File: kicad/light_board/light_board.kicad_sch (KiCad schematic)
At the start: 34 parts, among them J1 24V, J10 Screw_Terminal_01x02, J11 Screw_Terminal_01x02, J12 VAC, J13 NEUTRAL, J14 GND, J17 MCU_GND, J2 GND, J3 MCU_L1, J4 MCU_L2, J5 MCU_L3, J6 MCU_Bike, J7 MCU_5V, J8 Screw_Terminal_01x02, J9 Screw_Terminal_01x02, K1 1462041-7, Q1 FDD8453LZ, Q2 FDD8453LZ, Q4 FDD8453LZ, Q5 MOCD207M, Q6 MOCD207M

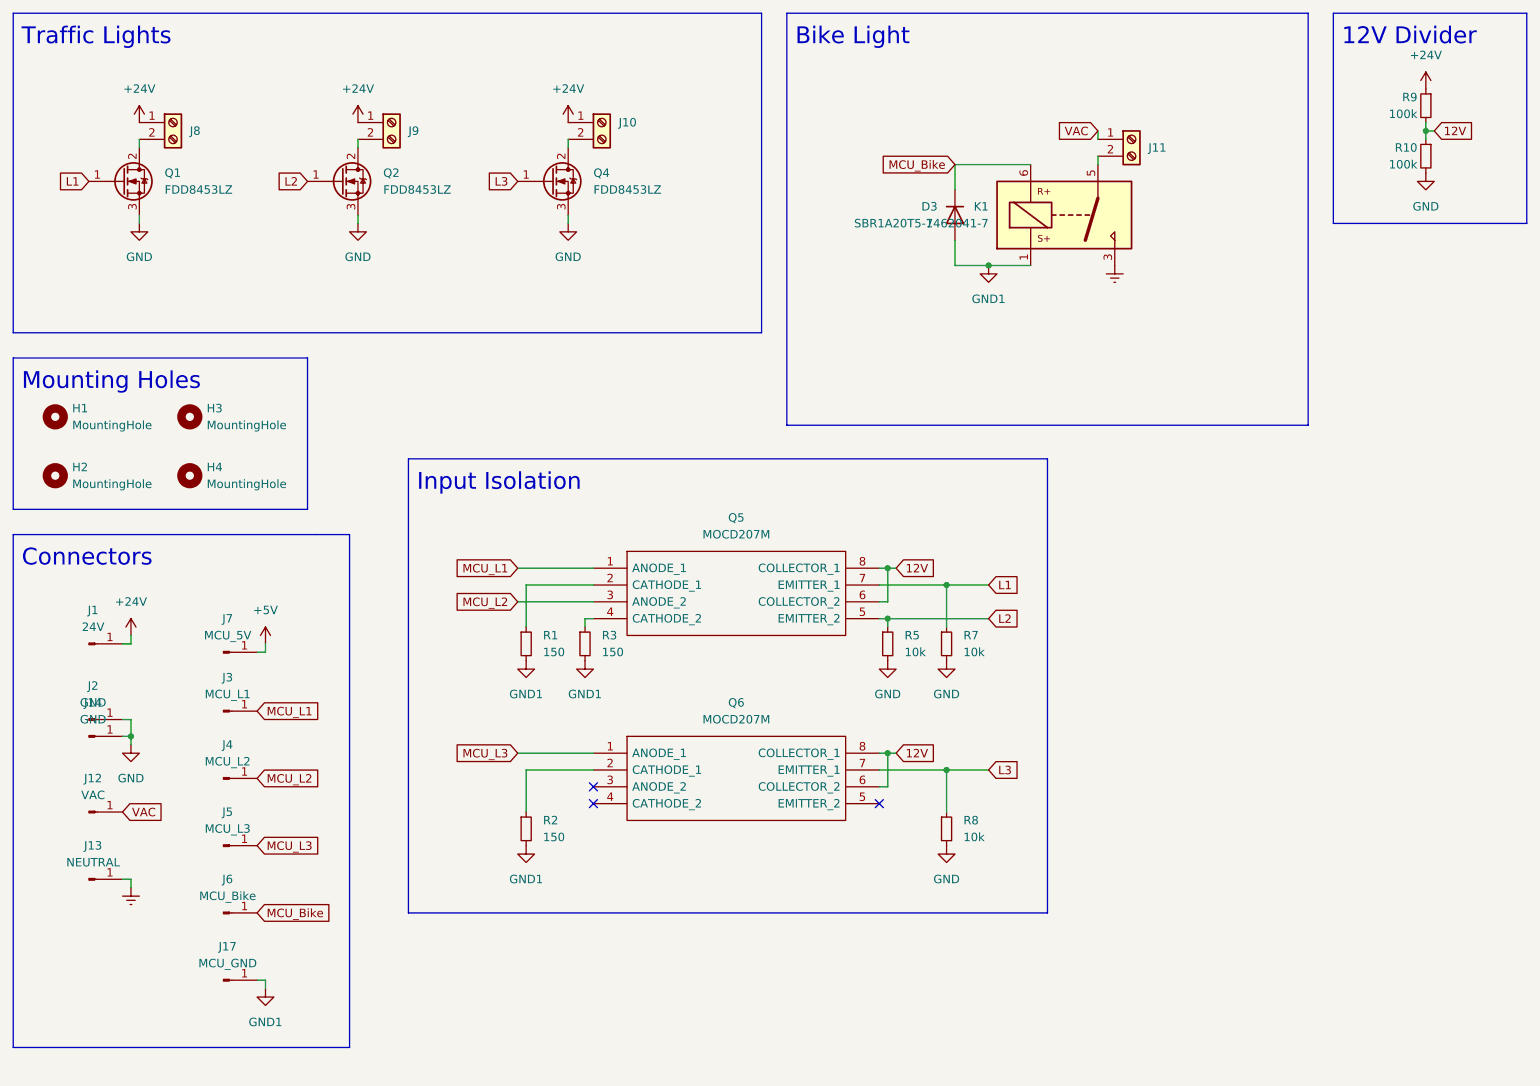
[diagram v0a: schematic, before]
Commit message: light board v2
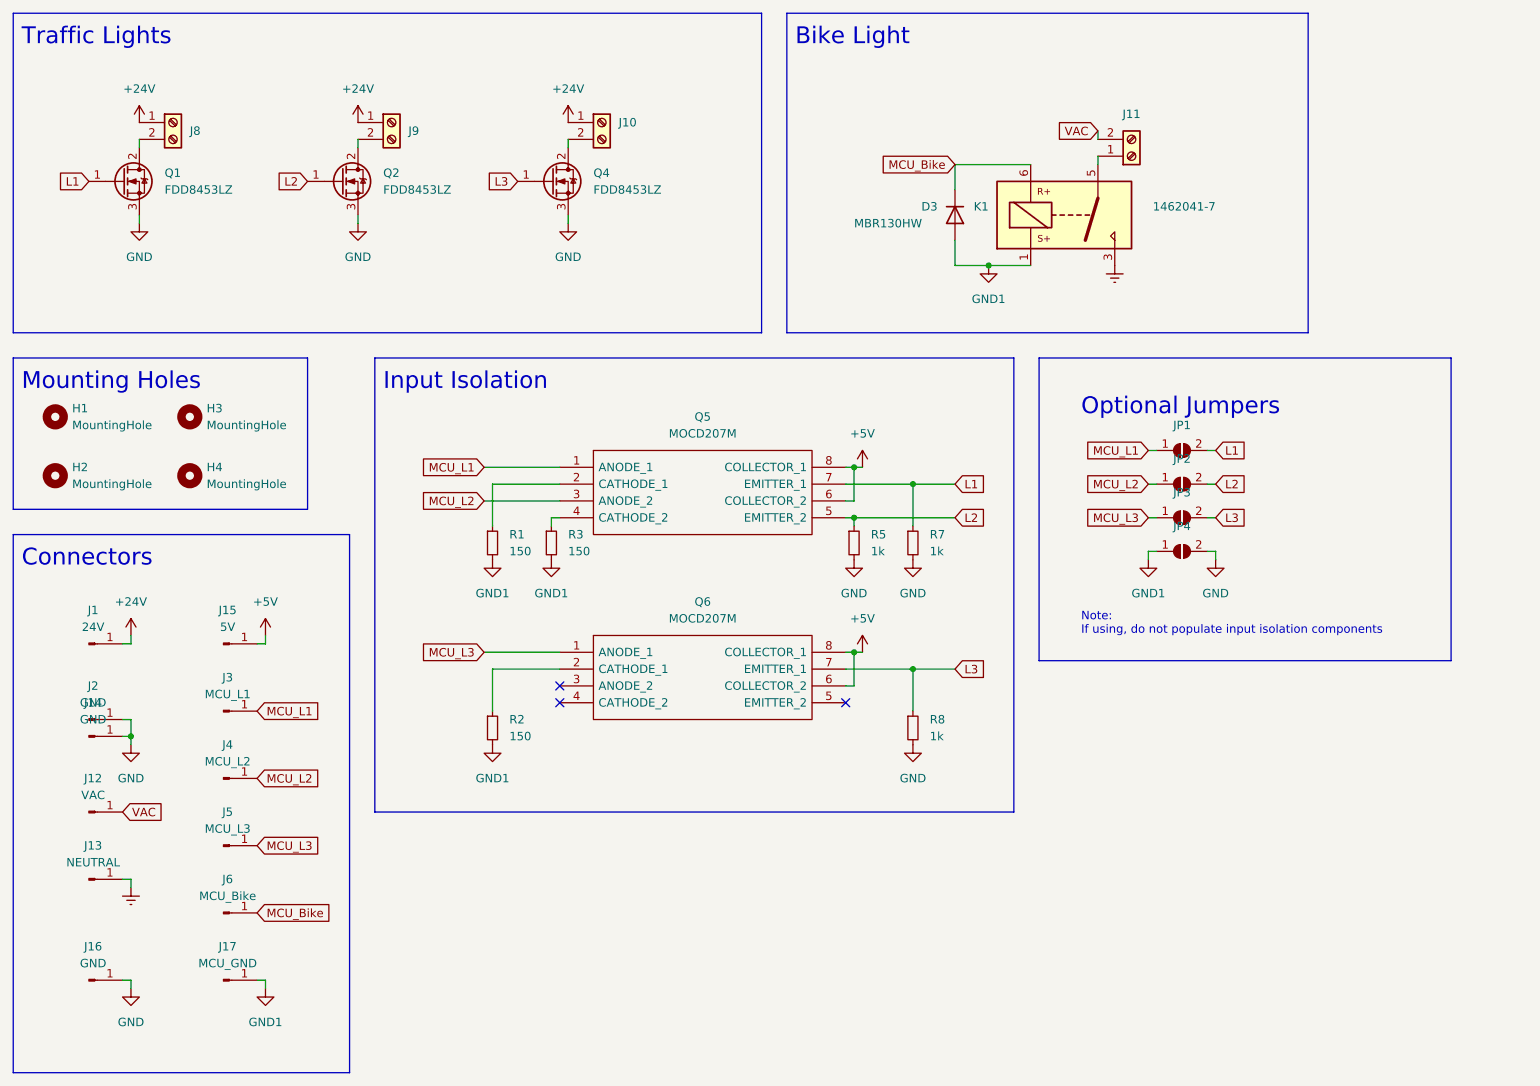
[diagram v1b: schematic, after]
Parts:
- removed J7: MCU_5V, Connector_PinHeader_2.54mm:PinHeader_1x01_P2.54mm_Vertical, symbol Connector:Conn_01x01_Male
- removed R10, R9: 100k, Resistor_SMD:R_1206_3216Metric, symbol Device:R_Small
- added J15: 5V, Connector_PinHeader_2.54mm:PinHeader_1x01_P2.54mm_Vertical, symbol Connector:Conn_01x01_Male
- added J16: GND, Connector_PinHeader_2.54mm:PinHeader_1x01_P2.54mm_Vertical, symbol Connector:Conn_01x01_Male
- added JP1, JP2, JP3, JP4: SolderJumper_2_Open, Jumper:SolderJumper-2_P1.3mm_Open_TrianglePad1.0x1.5mm, symbol Jumper:SolderJumper_2_Open
- D3: value SBR1A20T5-7 -> MBR130HW; footprint Diode_SMD:D_SOD-523 -> Diode_SMD:D_SOD-123
- R1, R2, R3: footprint Resistor_SMD:R_0805_2012Metric -> Resistor_SMD:R_0603_1608Metric
- R5, R7, R8: value 10k -> 1k; footprint Resistor_SMD:R_0805_2012Metric -> Resistor_SMD:R_0603_1608Metric
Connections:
- net 12V is gone; now on net +5V: Q5.6 (COLLECTOR_2), Q5.8 (COLLECTOR_1), Q6.6 (COLLECTOR_2), Q6.8 (COLLECTOR_1)
- net +5V: now also J15.1 (Pin_1)
- net GND: now also J16.1 (Pin_1), JP4.2 (B)
- net GND1: now also JP4.1 (A)
- net L1: now also JP1.2 (B)
- net L2: now also JP2.2 (B)
- net L3: now also JP3.2 (B)
- net MCU_L1: now also JP1.1 (A)
- net MCU_L2: now also JP2.1 (A)
- net MCU_L3: now also JP3.1 (A)
- net VAC: now also J11.2 (Pin_2); no longer J11.1 (Pin_1)
- net at K1.5: now also J11.1 (Pin_1); no longer J11.2 (Pin_2)
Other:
- note added: "Note: If using, do not populate input isolation components"
- note added: "Optional Jumpers"
- note removed: "12V Divider"
- moved on the sheet: Q5, Q6, R1, R2, R3, R5, R7, R8

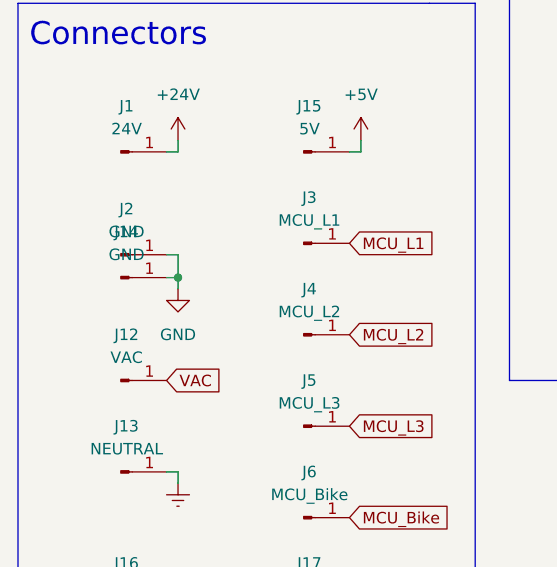
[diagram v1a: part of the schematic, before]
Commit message: update pcbs
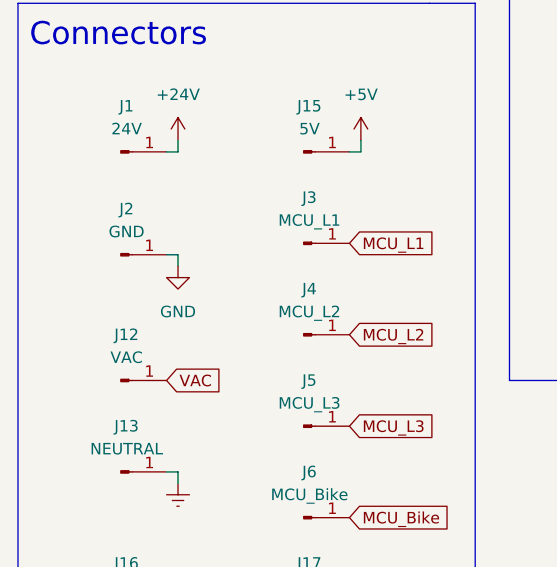
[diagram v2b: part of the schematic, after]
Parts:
- removed J14: GND, Connector_PinHeader_2.54mm:PinHeader_1x01_P2.54mm_Vertical, symbol Connector:Conn_01x01_Male
- J1, J12, J13, J2: footprint Connector_PinHeader_2.54mm:PinHeader_1x01_P2.54mm_Vertical -> _mylib:hole
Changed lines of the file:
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@@
   (junction (at 166.37 55.88) (diameter 0) (color 0 0 0 0)
-  )
-  (junction (at 36.83 127) (diameter 0) (color 0 0 0 0)
   )
   (junction (at 146.05 93.98) (diameter 0) (color 0 0 0 0)
@@
   (no_connect (at 144.78 121.92))
   (no_connect (at 101.6 119.38))
-  (wire (pts (xy 36.83 127) (xy 36.83 128.27))
-    (stroke (width 0) (type default) (color 0 0 0 0))
-  )
   (wire (pts (xy 146.05 86.36) (xy 144.78 86.36))
     (stroke (width 0) (type default) (color 0 0 0 0))
@@
     (stroke (width 0) (type default) (color 0 0 0 0))
   )
-  (wire (pts (xy 35.56 127) (xy 36.83 127))
-    (stroke (width 0) (type default) (color 0 0 0 0))
-  )
   (wire (pts (xy 146.05 93.98) (xy 146.05 95.25))
     (stroke (width 0) (type default) (color 0 0 0 0))
@@
     (stroke (width 0) (type default) (color 0 0 0 0))
   )
-  (wire (pts (xy 36.83 124.46) (xy 36.83 127))
+  (wire (pts (xy 36.83 124.46) (xy 36.83 125.73))
     (stroke (width 0) (type default) (color 0 0 0 0))
   )
@@
     (property "Reference" "J12" (id 0) (at 31.115 133.35 0))
     (property "Value" "VAC" (id 1) (at 31.115 135.89 0))
-    (property "Footprint" "Connector_PinHeader_2.54mm:PinHeader_1x01_P2.54mm_Vertical" (id 2) (at 30.48 138.43 0)
+    (property "Footprint" "_mylib:hole" (id 2) (at 30.48 138.43 0)
       (effects (font (size 1.27 1.27)) hide)
     )
@@
     (property "Reference" "J2" (id 0) (at 31.115 119.38 0))
     (property "Value" "GND" (id 1) (at 31.115 121.92 0))
-    (property "Footprint" "Connector_PinHeader_2.54mm:PinHeader_1x01_P2.54mm_Vertical" (id 2) (at 30.48 124.46 0)
+    (property "Footprint" "_mylib:hole" (id 2) (at 30.48 124.46 0)
       (effects (font (size 1.27 1.27)) hide)
     )
@@
     (property "Reference" "J1" (id 0) (at 31.115 107.95 0))
     (property "Value" "24V" (id 1) (at 31.115 110.49 0))
-    (property "Footprint" "Connector_PinHeader_2.54mm:PinHeader_1x01_P2.54mm_Vertical" (id 2) (at 30.48 113.03 0)
+    (property "Footprint" "_mylib:hole" (id 2) (at 30.48 113.03 0)
       (effects (font (size 1.27 1.27)) hide)
     )
@@
     (pin "1")
   )
-  (symbol (lib_id "power:GND") (at 36.83 128.27 0) (unit 1)
-    (in_bom yes) (on_board yes) (fields_autoplaced)
-    (property "Reference" "#PWR013" (id 0) (at 36.83 134.62 0)
-      (effects (font (size 1.27 1.27)) hide)
-    )
-    (property "Value" "GND" (id 1) (at 36.83 133.35 0))
-    (property "Footprint" "" (id 2) (at 36.83 128.27 0)
-      (effects (font (size 1.27 1.27)) hide)
-    )
-    (property "Datasheet" "" (id 3) (at 36.83 128.27 0)
+  (symbol (lib_id "power:GND") (at 36.83 125.73 0) (unit 1)
+    (in_bom yes) (on_board yes) (fields_autoplaced)
+    (property "Reference" "#PWR013" (id 0) (at 36.83 132.08 0)
+      (effects (font (size 1.27 1.27)) hide)
+    )
+    (property "Value" "GND" (id 1) (at 36.83 130.81 0))
+    (property "Footprint" "" (id 2) (at 36.83 125.73 0)
+      (effects (font (size 1.27 1.27)) hide)
+    )
+    (property "Datasheet" "" (id 3) (at 36.83 125.73 0)
       (effects (font (size 1.27 1.27)) hide)
     )
@@
     (property "Reference" "J13" (id 0) (at 31.115 143.51 0))
     (property "Value" "NEUTRAL" (id 1) (at 31.115 146.05 0))
-    (property "Footprint" "Connector_PinHeader_2.54mm:PinHeader_1x01_P2.54mm_Vertical" (id 2) (at 30.48 148.59 0)
+    (property "Footprint" "_mylib:hole" (id 2) (at 30.48 148.59 0)
       (effects (font (size 1.27 1.27)) hide)
     )
@@
     (pin "1")
     (pin "2")
-  )
-  (symbol (lib_id "Connector:Conn_01x01_Male") (at 30.48 127 0) (unit 1)
-    (in_bom yes) (on_board yes) (fields_autoplaced)
-    (property "Reference" "J14" (id 0) (at 31.115 121.92 0))
-    (property "Value" "GND" (id 1) (at 31.115 124.46 0))
-    (property "Footprint" "Connector_PinHeader_2.54mm:PinHeader_1x01_P2.54mm_Vertical" (id 2) (at 30.48 127 0)
-      (effects (font (size 1.27 1.27)) hide)
-    )
-    (property "Datasheet" "~" (id 3) (at 30.48 127 0)
-      (effects (font (size 1.27 1.27)) hide)
-    )
-    (pin "1")
   )
   (symbol (lib_id "_mine:MOCD207M") (at 101.6 86.36 0) (unit 1)
@@
     )
     (path "/3f03fd16-a09a-47f5-adca-50c300f3a91b"
-      (reference "J1") (unit 1) (value "24V") (footprint "Connector_PinHeader_2.54mm:PinHeader_1x01_P2.54mm_Vertical")
+      (reference "J1") (unit 1) (value "24V") (footprint "_mylib:hole")
     )
     (path "/2ebe7d52-7c41-4411-b9ef-dfc7a0409ee4"
-      (reference "J2") (unit 1) (value "GND") (footprint "Connector_PinHeader_2.54mm:PinHeader_1x01_P2.54mm_Vertical")
+      (reference "J2") (unit 1) (value "GND") (footprint "_mylib:hole")
     )
     (path "/6bc02308-6fbd-49c8-811d-539d13503d44"
@@
     )
     (path "/264d4db4-f564-46bd-9b21-cfd66b695585"
-      (reference "J12") (unit 1) (value "VAC") (footprint "Connector_PinHeader_2.54mm:PinHeader_1x01_P2.54mm_Vertical")
+      (reference "J12") (unit 1) (value "VAC") (footprint "_mylib:hole")
     )
     (path "/5378bcb6-accb-4c3e-aaff-ae0cd065931f"
-      (reference "J13") (unit 1) (value "NEUTRAL") (footprint "Connector_PinHeader_2.54mm:PinHeader_1x01_P2.54mm_Vertical")
-    )
-    (path "/c99e6d80-f2a9-415e-92b3-df98c4f485fa"
-      (reference "J14") (unit 1) (value "GND") (footprint "Connector_PinHeader_2.54mm:PinHeader_1x01_P2.54mm_Vertical")
+      (reference "J13") (unit 1) (value "NEUTRAL") (footprint "_mylib:hole")
     )
     (path "/385e0403-8b28-4505-873a-a91713d8181b"
